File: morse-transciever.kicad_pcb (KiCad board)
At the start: 2 copper layers, 49.5 x 28.5 mm, 42 parts, among them J1 Antenna connector, J2 jack_connecor, J3 PWR in, Q1 BC847, Q2 PZT2222AT1G, SW1 SW_Push, U1 LM386, Y1 3579 kHz

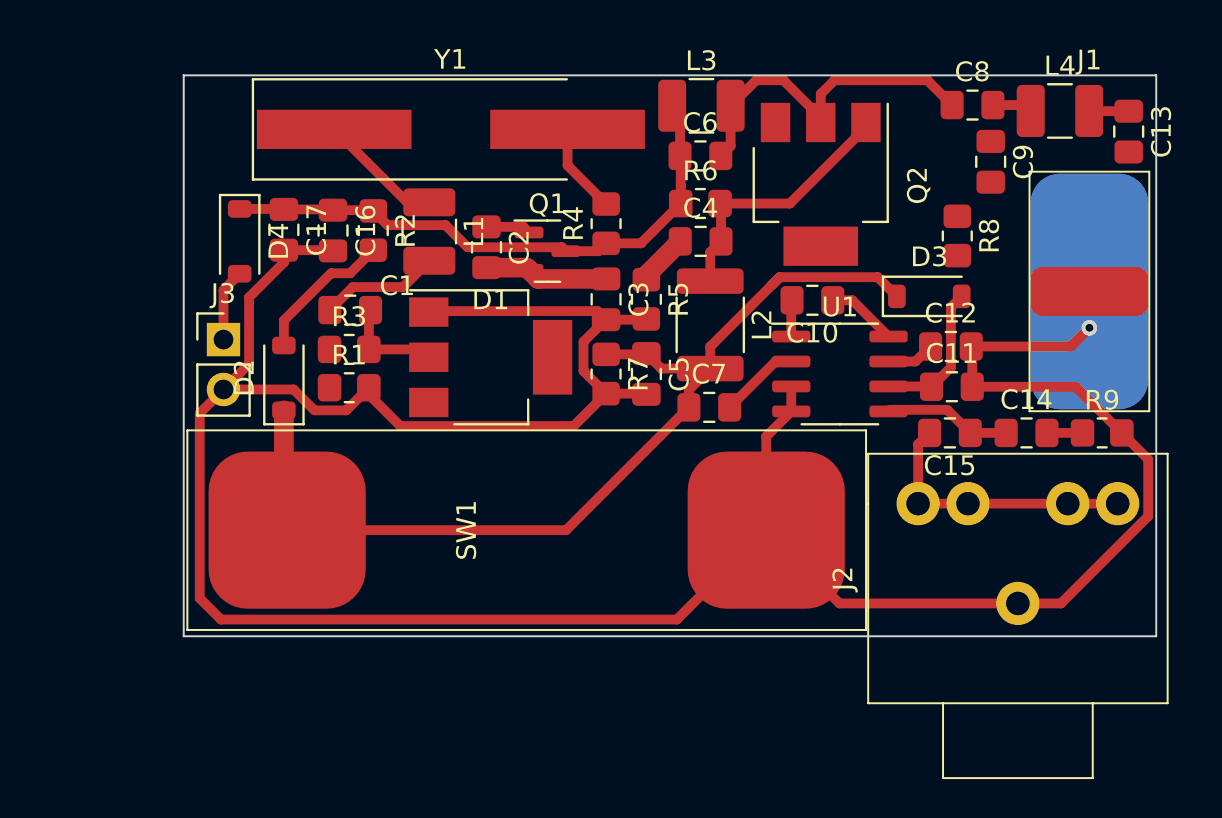
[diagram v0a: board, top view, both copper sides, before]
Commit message: Finalizing PCB design, ready for gerber generation
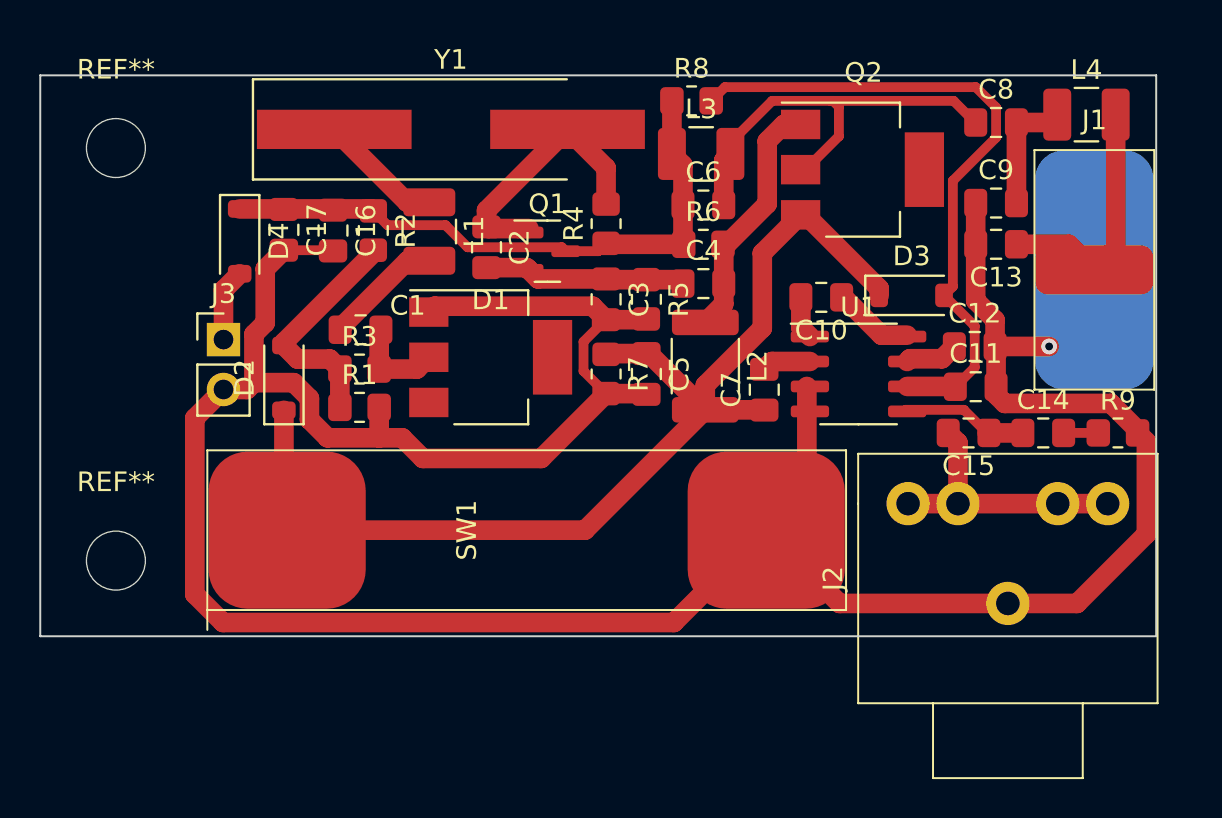
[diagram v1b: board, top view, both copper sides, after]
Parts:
- added REF**: MountingHole_3mm, MountingHole:MountingHole_3mm, F.Cu at (89.5, 81.0)
- added REF**: MountingHole_3mm, MountingHole:MountingHole_3mm, F.Cu at (89.5, 60.0)
- moved R8 15.2 mm to (118.8, 57.6), turned to 0 degrees
- moved C13 8.86 mm to (134.3, 64.9), turned to 180 degrees
- moved C7 2.94 mm to (122.5, 72.3), turned to 90 degrees
- moved C6 2.50 mm to (119.4, 62.9)
- moved L3 2.45 mm to (119.3, 60.3)
- moved Q2 2.25 mm to (127.5, 61.1), turned to 0 degrees
- moved C4 2.15 mm to (119.4, 66.9)
- moved C9 2.12 mm to (134.3, 62.8), turned to 0 degrees
- moved L2 2.11 mm to (119.5, 71.1)
- moved R6 2.08 mm to (119.4, 64.9)
- moved C8 1.49 mm to (134.3, 58.7)
- moved L4 1.36 mm to (138.9, 58.3)
- moved C12 1.21 mm to (133.2, 70.1)
- moved C11 1.21 mm to (133.3, 72.2)
- moved C1 1.13 mm to (102.0, 69.2)
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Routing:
- net Net-(D3-A): track 7.43 -> 34.0 mm
- net Net-(J1-In): track 2.02 -> 12.9 mm
- net GND: track 145.9 -> 153.1 mm
- net /audio: track 50.4 -> 57.2 mm
- net Net-(Q1-B): track 6.89 -> 13.5 mm
- net Net-(D2-A): track 7.59 -> 12.3 mm
- net Net-(C8-Pad2): track 2.08 -> 6.36 mm
- net /antenna: track 18.5 -> 21.7 mm
- net VCC: track 29.6 -> 31.3 mm
- net Net-(U1--): track 4.10 -> 2.49 mm
- net Net-(Q1-E): track 8.99 -> 10.3 mm
- net Net-(Q2-B): track 13.5 -> 12.7 mm
- net Net-(C10-Pad1): track 3.60 -> 4.13 mm
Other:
- board size 49.5 x 28.5 mm -> 56.8 x 28.5 mm
